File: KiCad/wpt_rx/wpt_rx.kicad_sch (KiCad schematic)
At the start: 28 parts, among them J1 Conn_Coaxial, U1 NCP1117-ADJ_SOT223

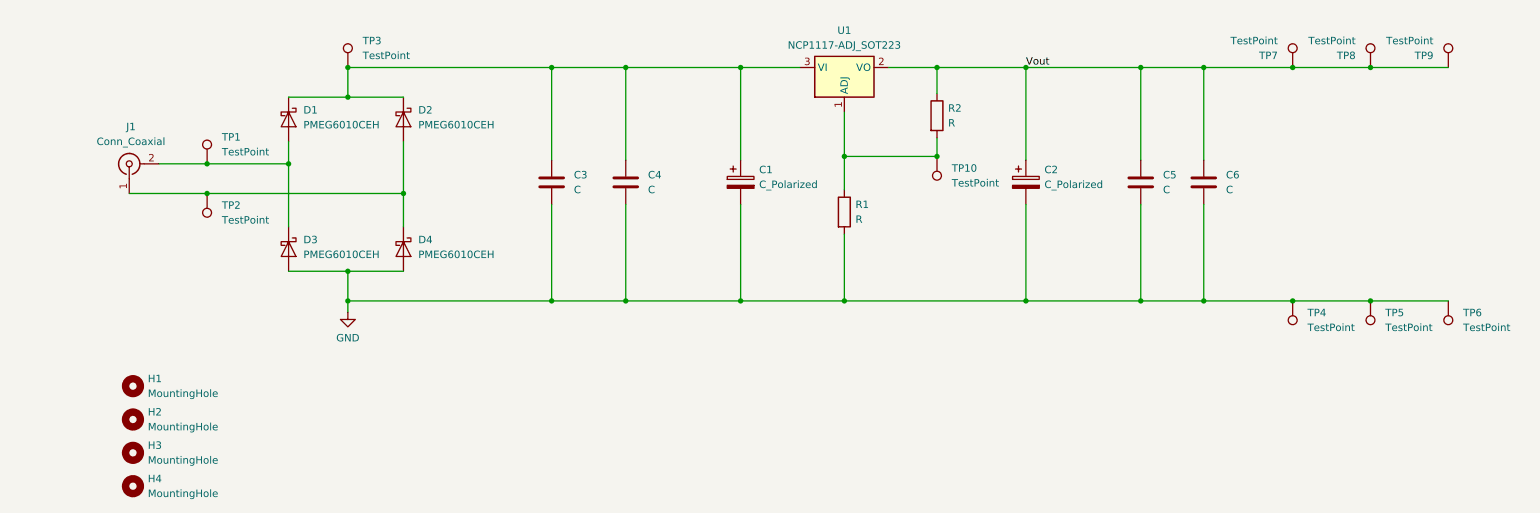
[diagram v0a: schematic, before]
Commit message: add file exports
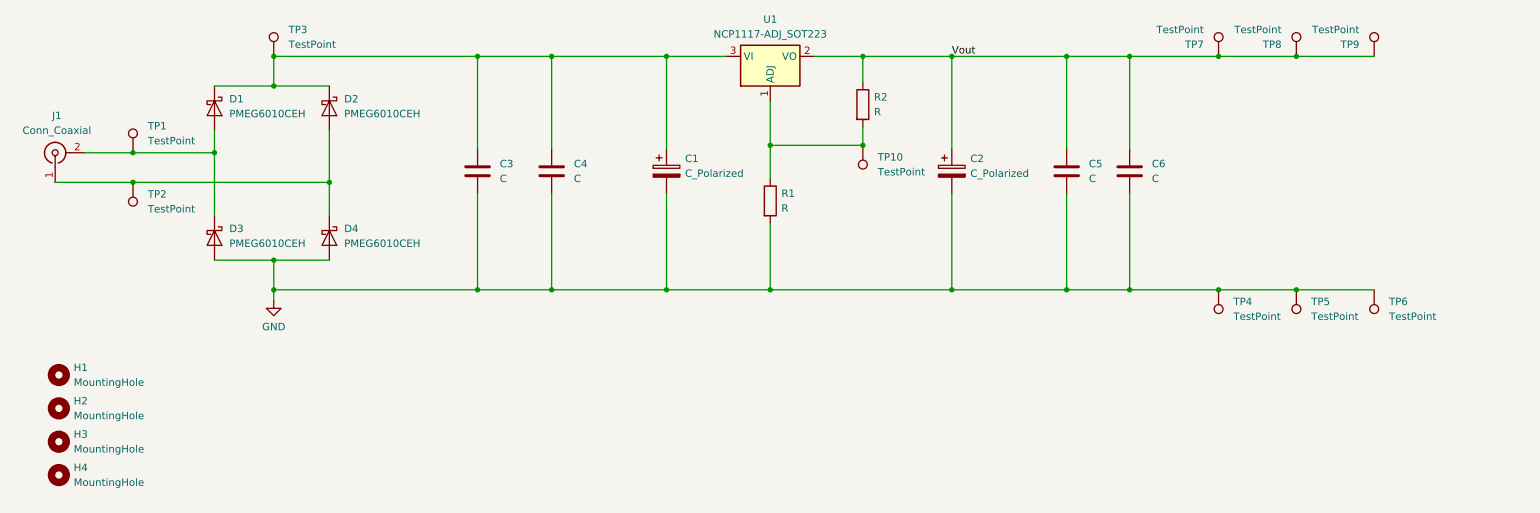
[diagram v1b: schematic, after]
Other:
- moved on the sheet: C1, C2, C3, C4, C5, C6, D1, D2, D3, D4, H1, H2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
